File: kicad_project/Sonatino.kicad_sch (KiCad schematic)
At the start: 35 parts, among them J2 Conn_02x09_Odd_Even, SW1 SW_Push, SW2 SW_Push, SW3 SW_DIP_x02, U2 ESP32-S3-WROOM-1U

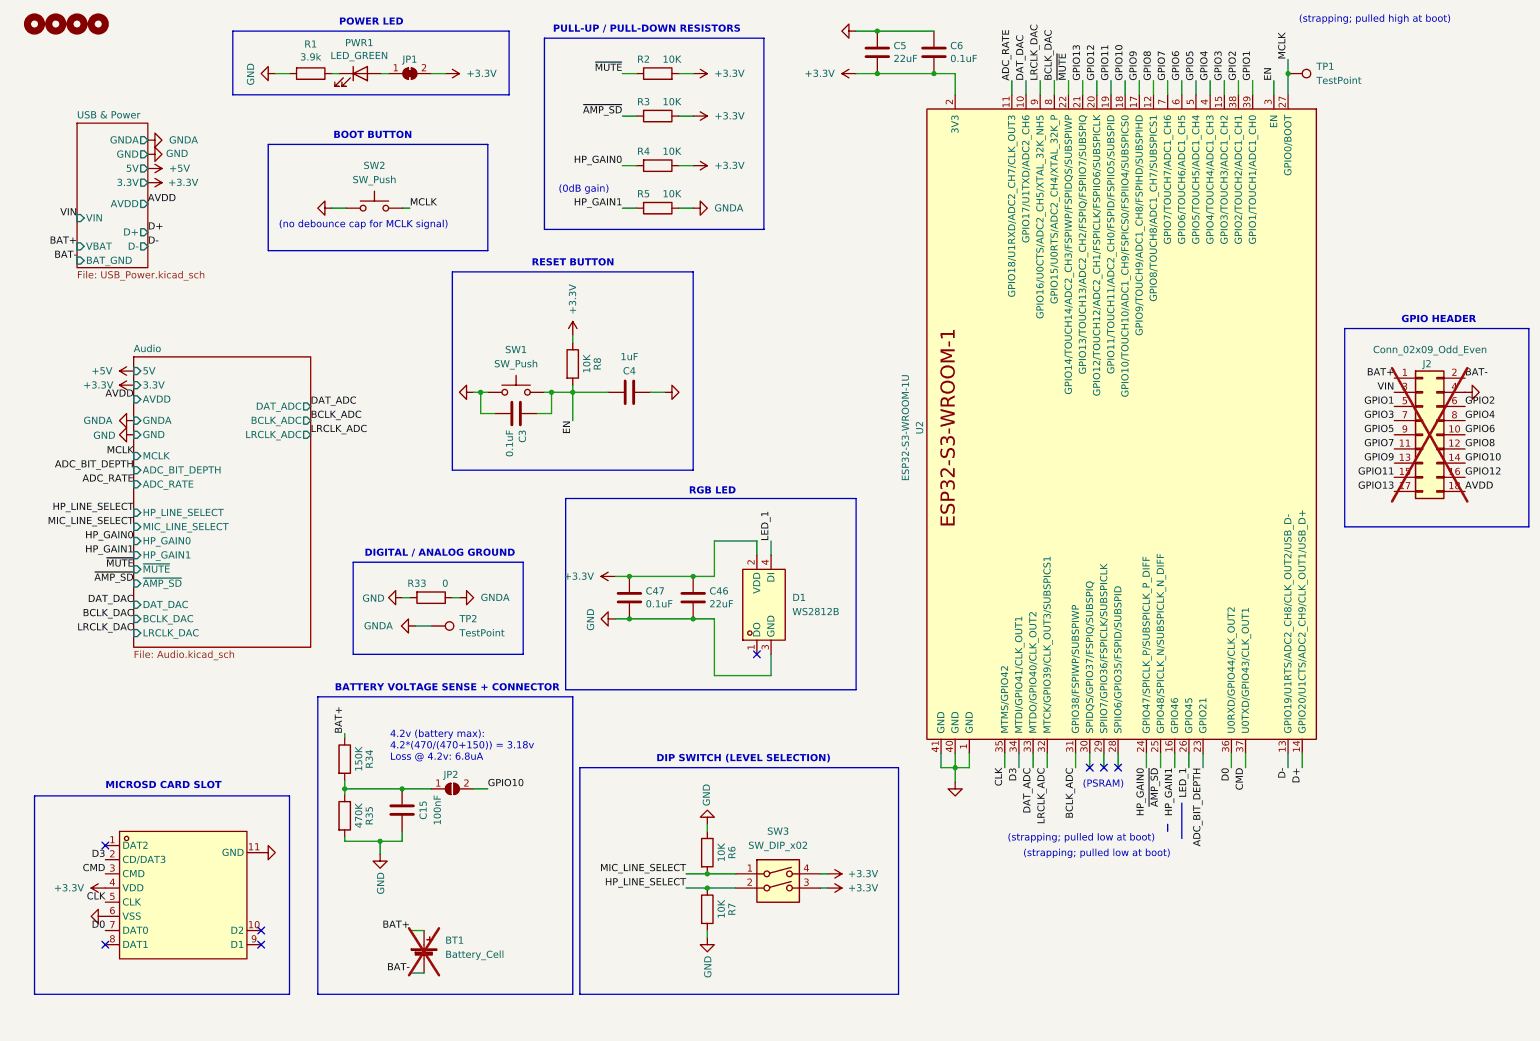
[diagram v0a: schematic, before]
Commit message: Initial commit
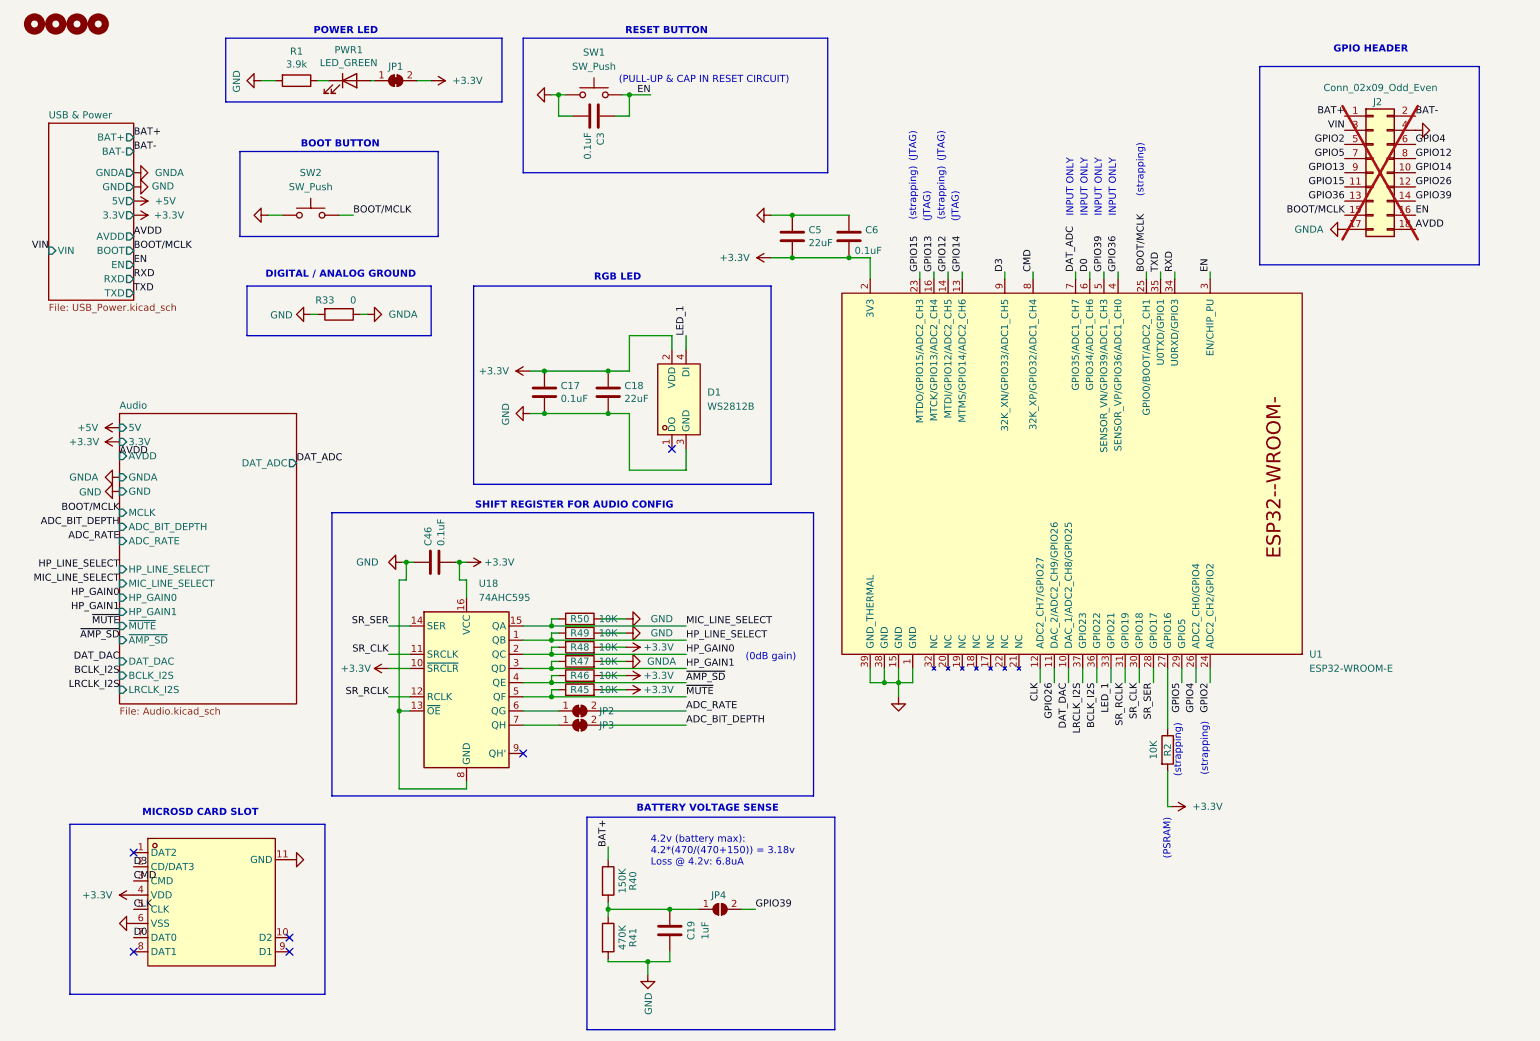
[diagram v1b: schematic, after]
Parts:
- removed BT1: Battery_Cell, Connector_JST:JST_PH_S2B-PH-SM4-TB_1x02-1MP_P2.00mm_Horizontal, symbol Device:Battery_Cell
- removed C15: 100nF, Capacitor_SMD:C_0402_1005Metric, symbol Device:C
- removed C4: 1uF, Capacitor_SMD:C_0402_1005Metric, symbol Device:C
- removed C47: 0.1uF, Capacitor_SMD:C_0402_1005Metric, symbol Device:C
- removed Card2: TF-008, Custom:TF-SMD_TF-008, symbol Custom:TF-008
- removed JP2: SolderJumper_2_Open, Jumper:SolderJumper-2_P1.3mm_Open_TrianglePad1.0x1.5mm, symbol Jumper:SolderJumper_2_Open
- removed R3, R4, R5, R6, R7, R8: 10K, Resistor_SMD:R_0402_1005Metric, symbol Device:R
- removed R34: 150K, Resistor_SMD:R_0402_1005Metric, symbol Device:R
- removed R35: 470K, Resistor_SMD:R_0402_1005Metric, symbol Device:R
- removed SW3: SW_DIP_x02, Button_Switch_SMD:SW_DIP_SPSTx02_Slide_Omron_A6H-2101_W6.15mm_P1.27mm, symbol Switch:SW_DIP_x02
- removed TP1, TP2: TestPoint, TestPoint:TestPoint_Pad_D1.5mm, symbol Connector:TestPoint
- removed U2: ESP32-S3-WROOM-1U, Espressif:ESP32-S3-WROOM-1U, symbol Espressif:ESP32-S3-WROOM-1
- added C17: 0.1uF, Capacitor_SMD:C_0402_1005Metric, symbol Device:C
- added C18: 22uF, Capacitor_SMD:C_0603_1608Metric, symbol Device:C
- added C19: 1uF, Capacitor_SMD:C_0402_1005Metric, symbol Device:C
- added Card1: TF-008, Custom:TF-SMD_TF-008, symbol Custom:TF-008
- added JP2, JP3: SolderJumper_2_Bridged, Jumper:SolderJumper-2_P1.3mm_Bridged_Pad1.0x1.5mm, symbol Jumper:SolderJumper_2_Bridged
- added JP4: SolderJumper_2_Open, Jumper:SolderJumper-2_P1.3mm_Open_TrianglePad1.0x1.5mm, symbol Jumper:SolderJumper_2_Open
- added R40: 150K, Resistor_SMD:R_0402_1005Metric, symbol Device:R
- added R41: 470K, Resistor_SMD:R_0402_1005Metric, symbol Device:R
- added R45, R46, R47, R48, R49, R50: 10K, Resistor_SMD:R_0402_1005Metric, symbol Device:R
- added U1: ESP32-WROOM-E, Espressif:ESP32-WROOM-32UE, symbol Espressif:ESP32-WROOM-E
- added U18: 74AHC595, Custom:X1-QFN-16-EP_L2.5-W2.5-P0.40-BL-EP1.4, symbol 74xx:74AHC595
- C46: value 22uF -> 0.1uF; footprint Capacitor_SMD:C_0805_2012Metric -> Capacitor_SMD:C_0402_1005Metric; LCSC C45783 -> C307331
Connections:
- net GPIO1 is gone; now on net GPIO2: J2.5 (Pin_5)
- net GPIO3 is gone; now on net GPIO5: J2.7 (Pin_7)
- net MCLK is gone; now on net BOOT/MCLK: SW2.2
- net +3.3V: now also C46.2, C17.1, C18.1, Card1.4 (VDD), R45.2, R46.2, R48.2, U1.2 (3V3), U18.10 (~{SRCLR}), U18.16 (VCC); no longer C46.1
- net ADC_BIT_DEPTH: now also JP3.2 (B)
- net ADC_RATE: now also JP2.2 (B)
- net BAT+: now also R40.1
- net CLK: now also Card1.5 (CLK), U1.12 (ADC2_CH7/GPIO27)
- net CMD: now also Card1.3 (CMD), U1.8 (32K_XP/GPIO32/ADC1_CH4)
- net D0: now also Card1.7 (DAT0), U1.6 (GPIO34/ADC1_CH6)
- net D3: now also Card1.2 (CD/DAT3), U1.9 (32K_XN/GPIO33/ADC1_CH5)
- net DAT_ADC: now also U1.7 (GPIO35/ADC1_CH7)
- net DAT_DAC: now also U1.10 (DAC_1/ADC2_CH8/GPIO25)
- net EN: now also J2.16 (Pin_16), U1.3 (EN/CHIP_PU)
- net GND: now also C46.1, C17.2, C18.2, C19.1, Card1.11 (GND), Card1.6 (VSS), R41.2, R49.2, R50.2, U1.1 (GND), U1.15 (GND), U1.38 (GND), U1.39 (GND_THERMAL), U18.13 (~{OE}), U18.8 (GND); no longer C46.2
- net GNDA: now also J2.17 (Pin_17), R47.2
- net GPIO12: now also J2.8 (Pin_8), U1.14 (MTDI/GPIO12/ADC2_CH5); no longer J2.16 (Pin_16)
- net GPIO13: now also J2.9 (Pin_9), U1.16 (MTCK/GPIO13/ADC2_CH4); no longer J2.17 (Pin_17)
- net GPIO2: now also U1.24 (ADC2_CH2/GPIO2); no longer J2.6 (Pin_6)
- net GPIO4: now also J2.6 (Pin_6), U1.26 (ADC2_CH0/GPIO4); no longer J2.8 (Pin_8)
- net GPIO5: now also U1.29 (GPIO5); no longer J2.9 (Pin_9)
- net HP_GAIN0: now also R48.1, U18.2 (QC)
- net HP_GAIN1: now also R47.1, U18.3 (QD)
- net HP_LINE_SELECT: now also R49.1, U18.1 (QB)
- net LED_1: now also U1.33 (GPIO21)
- net MIC_LINE_SELECT: now also R50.1, U18.15 (QA)
- net ~{AMP_SD}: now also R46.1, U18.4 (QE)
- net ~{MUTE}: now also R45.1, U18.5 (QF); no longer R2.1
- net GPIO10 renamed GPIO39
- net GPIO39: now also JP4.2 (B), U1.5 (SENSOR_VN/GPIO39/ADC1_CH3)
- net GPIO11 renamed BOOT/MCLK
- net BOOT/MCLK: now also U1.25 (GPIO0/BOOT/ADC2_CH1)
- net GPIO6 renamed GPIO14
- net GPIO14: now also U1.13 (MTMS/GPIO14/ADC2_CH6)
- net GPIO7 renamed GPIO15
- net GPIO15: now also U1.23 (MTDO/GPIO15/ADC2_CH3)
- net GPIO8 renamed GPIO26
- net GPIO26: now also U1.11 (DAC_2/ADC2_CH9/GPIO26)
- net GPIO9 renamed GPIO36
- net GPIO36: now also U1.4 (SENSOR_VP/GPIO36/ADC1_CH0)
- new net: JP2.1 (A), U18.6 (QG)
- new net: C19.2, JP4.1 (A), R40.2, R41.1
- new net: R2.1, U1.27 (GPIO16)
- new net: JP3.1 (A), U18.7 (QH)
- new net BCLK_I2S: U1.36 (GPIO22)
- new net LRCLK_I2S: U1.37 (GPIO23)
- new net RXD: U1.34 (U0RXD/GPIO3)
- new net SR_CLK: U1.30 (GPIO18), U18.11 (SRCLK)
- new net SR_RCLK: U1.31 (GPIO19), U18.12 (RCLK)
- new net SR_SER: U1.28 (GPIO17), U18.14 (SER)
- new net TXD: U1.35 (U0TXD/GPIO1)
- no-connect marks 8 -> 6
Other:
- sheet Audio ports: added BCLK_I2S, LRCLK_I2S; removed BCLK_ADC, BCLK_DAC, LRCLK_ADC, LRCLK_DAC
- sheet USB & Power ports: added BAT+, BAT-, BOOT, EN, RXD, TXD; removed BAT_GND, D+, D-, VBAT
- note added: "(JTAG)"
- note added: "(PULL-UP & CAP IN RESET CIRCUIT)"
- note added: "(strapping)"
- note added: "BATTERY VOLTAGE SENSE"
- note added: "INPUT ONLY"
- note added: "SHIFT REGISTER FOR AUDIO CONFIG"
- note removed: "(no debounce cap for MCLK signal)"
- note removed: "(strapping; pulled high at boot)"
- note removed: "(strapping; pulled low at boot)"
- note removed: "BATTERY VOLTAGE SENSE + CONNECTOR"
- note removed: "DIP SWITCH (LEVEL SELECTION)"
- note removed: "PULL-UP / PULL-DOWN RESISTORS"
- title: Sonatino -> Sonatino - Bluetooth Audio Edition
- moved on the sheet: C3, C5, C6, J2, JP1, PWR1, R1, R33, SW1, SW2
